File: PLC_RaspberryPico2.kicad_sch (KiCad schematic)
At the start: 26 parts, among them J1 Salidas Digitales a Reles, J10 ID1, J11 Alimentacion, J12 ID2, J2 ID1, J3 ID2, J4 ID3, J5 ID4, J6 ID5, J7 ID6, J8 ID7, J9 ID8, SW1 SW_Push, SW2 SW_Push, SW3 SW_Push, SW4 SW_Push

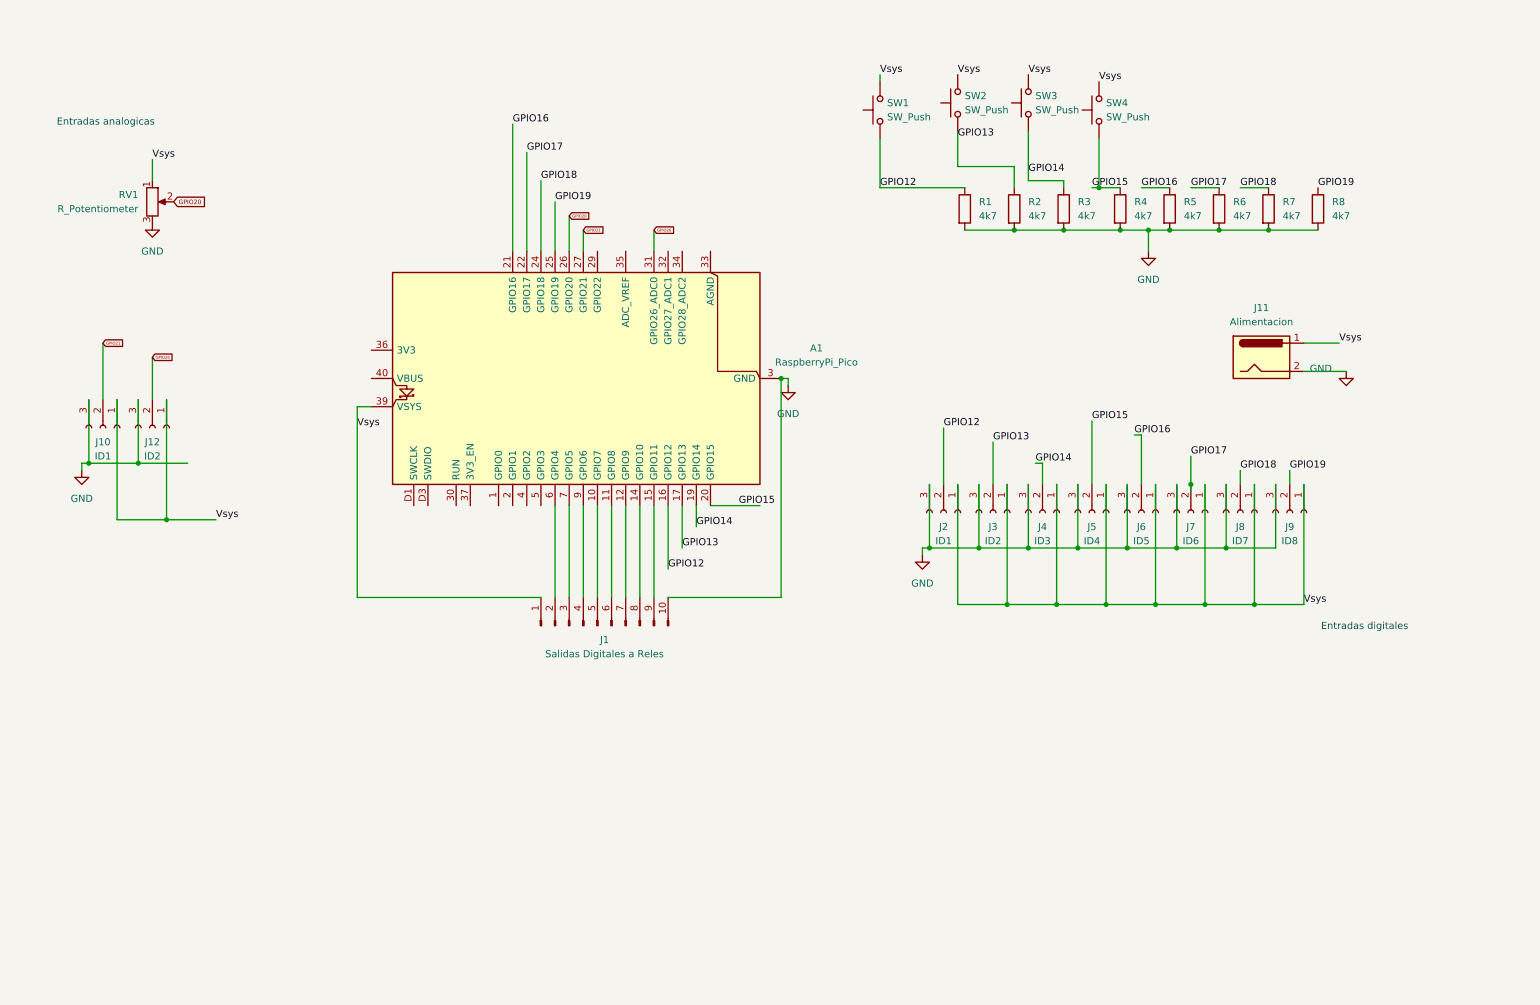
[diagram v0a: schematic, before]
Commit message: 2 de Octubre
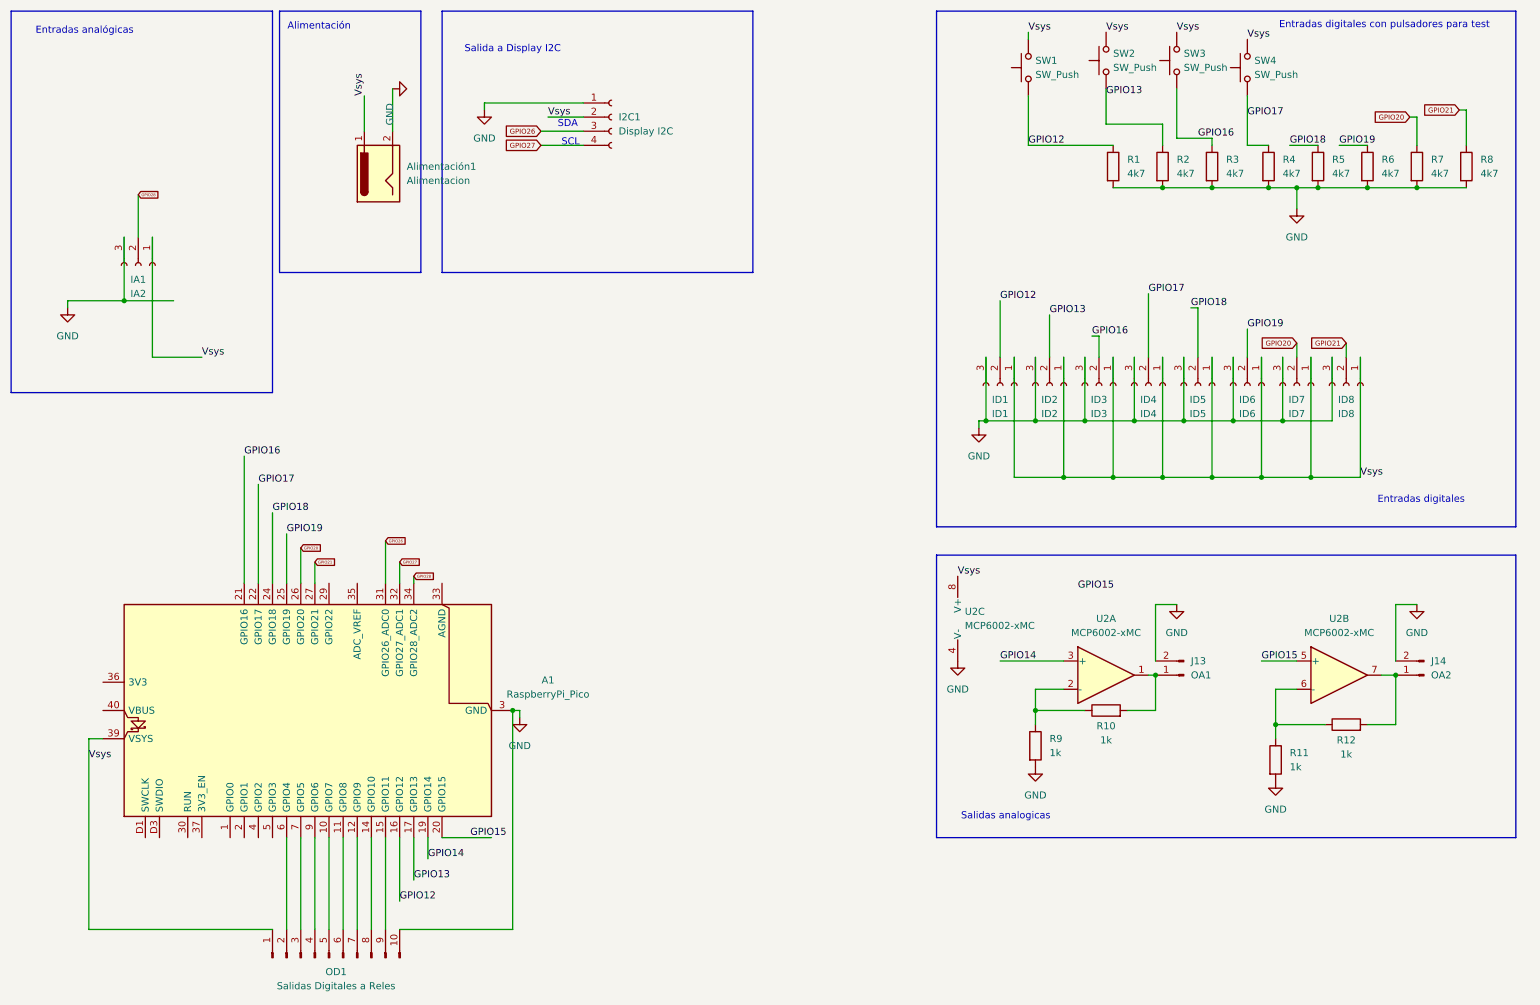
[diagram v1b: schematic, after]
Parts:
- removed J10: ID1, TerminalBlock:TerminalBlock_MaiXu_MX126-5.0-03P_1x03_P5.00mm, symbol Connector:Conn_01x03_Socket
- removed RV1: R_Potentiometer, symbol Device:R_Potentiometer
- added I2C1: Display I2C, Connector_PinHeader_2.54mm:PinHeader_1x04_P2.54mm_Vertical, symbol Connector:Conn_01x04_Socket
- added J13: OA1, TerminalBlock:TerminalBlock_MaiXu_MX126-5.0-02P_1x02_P5.00mm, symbol Connector:Conn_01x02_Pin
- added J14: OA2, TerminalBlock:TerminalBlock_MaiXu_MX126-5.0-02P_1x02_P5.00mm, symbol Connector:Conn_01x02_Pin
- added R10, R11, R12, R9: 1k, Resistor_THT:R_Axial_DIN0204_L3.6mm_D1.6mm_P7.62mm_Horizontal, symbol Device:R
- added U2: MCP6002-xMC, Package_DIP:DIP-8_W7.62mm_Socket_LongPads, symbol Amplifier_Operational:MCP6002-xMC
- A1: footprint Module:RaspberryPi_Pico_SMD_HandSolder -> Module:RaspberryPi_Pico_Common_THT
- Alimentación1: renamed from J11; footprint Connector_BarrelJack:BarrelJack_Horizontal -> Connector_BarrelJack:BarrelJack_CUI_PJ-079BH_Horizontal
- IA1: renamed from J12; value ID2 -> IA2
- renumbered J2 to ID1, J3 to ID2, J4 to ID3, J5 to ID4, J6 to ID5, J7 to ID6, J8 to ID7, J9 to ID8, J1 to OD1
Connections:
- net GND: now also I2C1.1 (Pin_1), J13.2 (Pin_2), J14.2 (Pin_2), R11.2, R9.2, U2.4 (V-), U2.9 (V-)
- net GPIO14: now also U2.3 (+); no longer ID3.2 (Pin_2), R3.1, SW3.1
- net GPIO15: now also U2.5 (+); no longer ID4.2 (Pin_2), R4.1, SW4.1
- net GPIO16: now also ID3.2 (Pin_2), R3.1, SW3.1; no longer ID5.2 (Pin_2), R5.1
- net GPIO17: now also ID4.2 (Pin_2), R4.1, SW4.1; no longer ID6.2 (Pin_2), R6.1
- net GPIO18: now also ID5.2 (Pin_2), R5.1; no longer ID7.2 (Pin_2), R7.1
- net GPIO19: now also ID6.2 (Pin_2), R6.1; no longer ID8.2 (Pin_2), R8.1
- net GPIO20: now also ID7.2 (Pin_2), R7.1
- net GPIO21: now also ID8.2 (Pin_2), R8.1
- net GPIO26: now also I2C1.3 (Pin_3); no longer IA1.2 (Pin_2)
- net Vsys: now also I2C1.2 (Pin_2), U2.8 (V+)
- net GPIO27: now reaches A1.32 (GPIO27_ADC1)
- net GPIO27: now also I2C1.4 (Pin_4)
- net GPIO28: now reaches A1.34 (GPIO28_ADC2)
- net GPIO28: now also IA1.2 (Pin_2)
- new net: J13.1 (Pin_1), R10.2, U2.1
- new net: R10.1, R9.1, U2.2 (-)
- new net: R11.1, R12.1, U2.6 (-)
- new net: J14.1 (Pin_1), R12.2, U2.7
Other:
- note added: "Alimentación"
- note added: "Entradas analógicas"
- note added: "Entradas digitales con pulsadores para test"
- note added: "SCL"
- note added: "SDA"
- note added: "Salida a Display I2C"
- note added: "Salidas analogicas"
- note removed: "Entradas analogicas"
- title: (none) -> Placa OPEN-PLC-Pico2
- moved on the sheet: A1, Alimentación1, IA1, ID1, ID2, ID3, ID4, ID5, ID6, ID7, ID8, OD1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
